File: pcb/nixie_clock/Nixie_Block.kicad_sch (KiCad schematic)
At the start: 25 parts, among them U66 MSD42WT1G, U67 MSD42WT1G, U68 MSD42WT1G, U69 MSD42WT1G, U70 MSD42WT1G, U71 MSD42WT1G, U72 MSD42WT1G, U73 MSD42WT1G, U74 MSD42WT1G, U75 MSD42WT1G, U76 MSD42WT1G, U77 MSD42WT1G

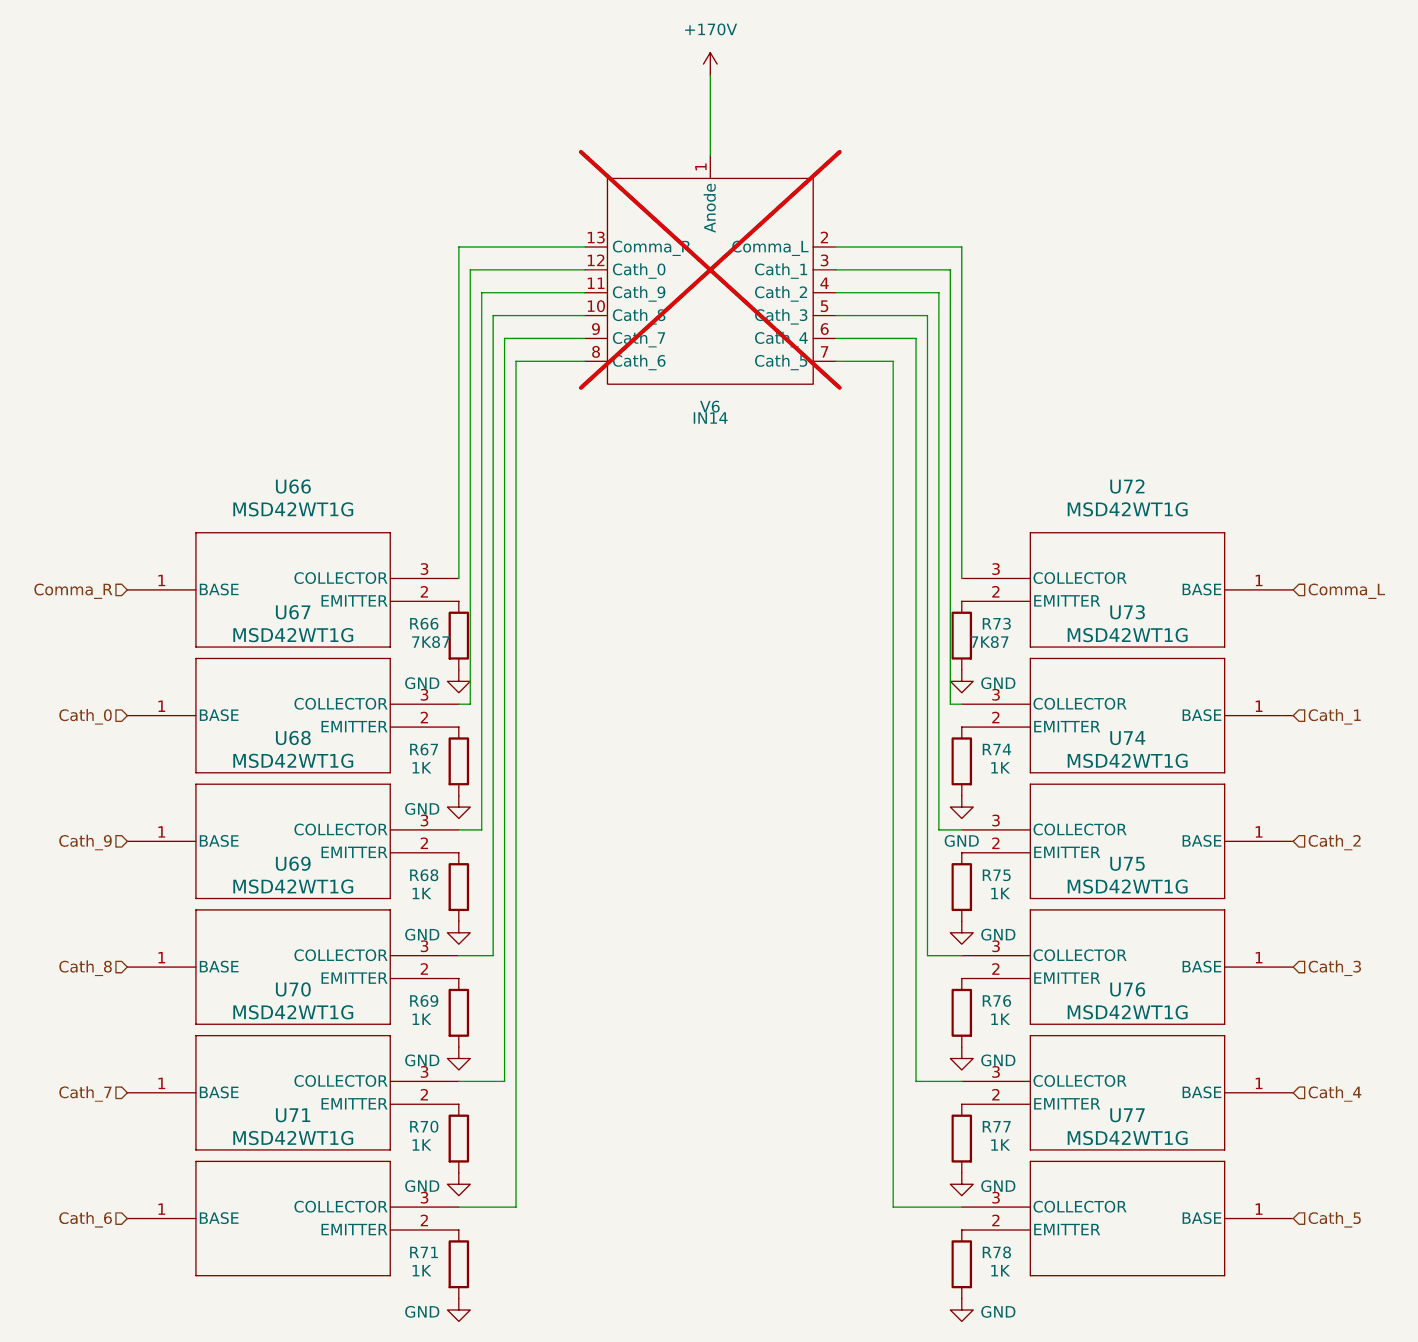
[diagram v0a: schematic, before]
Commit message: added grounding
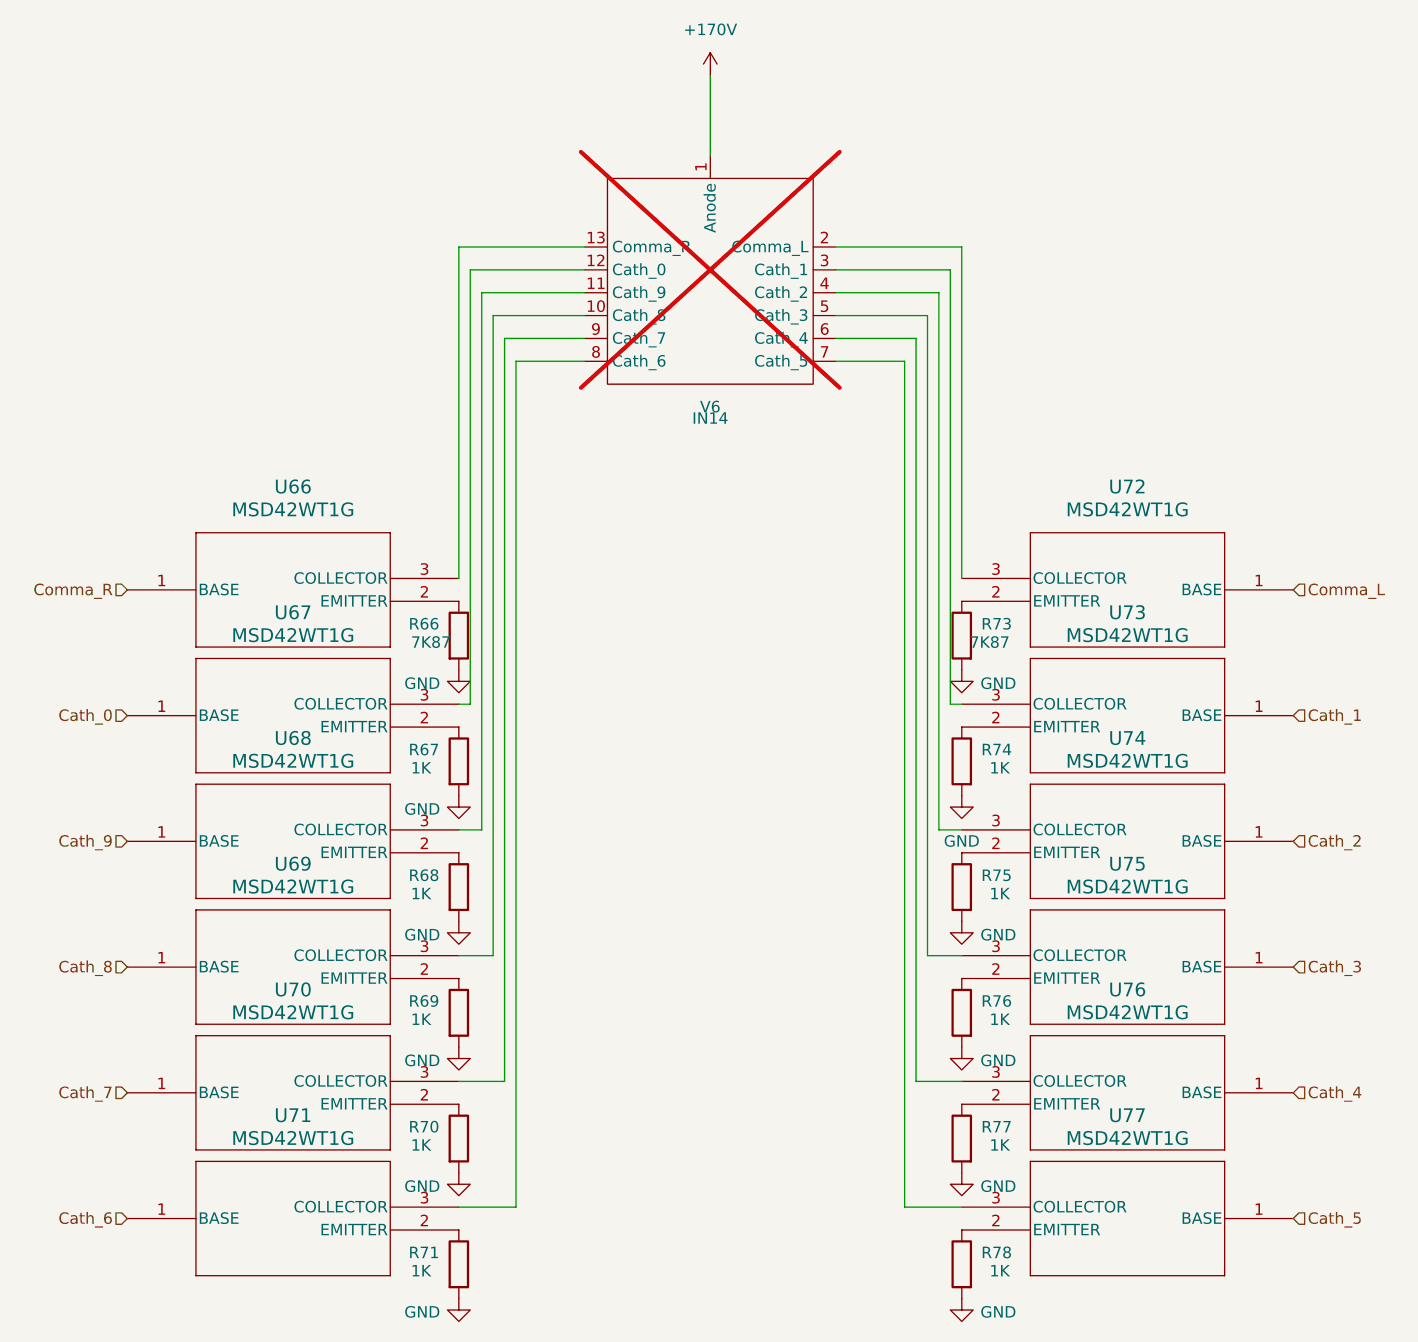
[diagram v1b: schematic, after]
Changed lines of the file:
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@@
 	(wire
 		(pts
-			(xy 129.54 160.02) (xy 121.92 160.02)
+			(xy 129.54 160.02) (xy 123.19 160.02)
 		)
 		(stroke
@@
 	(wire
 		(pts
-			(xy 121.92 160.02) (xy 121.92 66.04)
+			(xy 123.19 160.02) (xy 123.19 66.04)
 		)
 		(stroke
@@
 	(wire
 		(pts
-			(xy 121.92 66.04) (xy 115.57 66.04)
+			(xy 123.19 66.04) (xy 115.57 66.04)
 		)
 		(stroke
